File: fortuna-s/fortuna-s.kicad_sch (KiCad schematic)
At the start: 44 parts, among them J1 Ext Pinout, J2 Conn_01x21, J3 Conn_01x21, J6 Power (to panel), U1 74HTC138, U2 74HTC175

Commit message: .
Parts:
- removed C1, C2, C? (x4): 10uF, symbol Device:C
- removed J1: Ext Pinout, symbol Connector_Generic:Conn_02x13_Counter_Clockwise
- removed J2, J3: Conn_01x21, symbol Connector_Generic:Conn_01x21
- removed J?: FTDI cable, symbol Connector_Generic:Conn_01x06
- removed R? (x4): 10K, symbol Device:R_US
- removed R?: 3k3, symbol Device:R_US
- removed U1: 74HTC138, symbol 74xx:74LS138
- removed U2: 74HTC175, symbol 74xx:74LS175
- removed U? (x4): 74LS32, symbol 74xx:74LS32
- removed U?: 28C256, symbol Memory_EEPROM:28C256
- removed U?: AS6C4008-55PCN, Package_DIP:DIP-32_W15.24mm, symbol Memory_RAM:AS6C4008-55PCN
- removed U?: MC68B50, Package_DIP:DIP-40_W15.24mm, symbol Interface_UART:MC68B50
- removed U? (x2): 74HCT04, symbol 74xx:74HCT04
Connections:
- net VCC: no longer P?.A4 (VBUS), P?.A9 (VBUS), P?.B4 (VBUS), P?.B9 (VBUS), SW?.1
- net CLK_UART renamed CLK_EXT
- new net 5V_FTDI: P?.A4 (VBUS), P?.A9 (VBUS), P?.B4 (VBUS), P?.B9 (VBUS), SW?.1
- no-connect marks 18 -> 7
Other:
- added sheet Memory (memory.kicad_sch)
- added sheet Peripheral (peripheral.kicad_sch)
- note removed: "0x80 - Write serial 0x81 - Read serial"
- note removed: "BANKSWITCHING"
- note removed: "DEBUGGER"
- note removed: "EXTERNAL I/O"
- note removed: "I/O MULTIPLEXER"
- note removed: "IO address: write to 0x0"
- note removed: "MEMORY"
- note removed: "Occupies 0x80 to 0xBF in memory map."
- note removed: "The computer can be powered by the FTDI cable, but current can't exceed 350 mA."
- note removed: "UART"
- note removed: "UART communcates at 115000 baud."
- moved on the sheet: C?, D?, J6, JP1, JP?, P?, R?, SW?, U?, X?

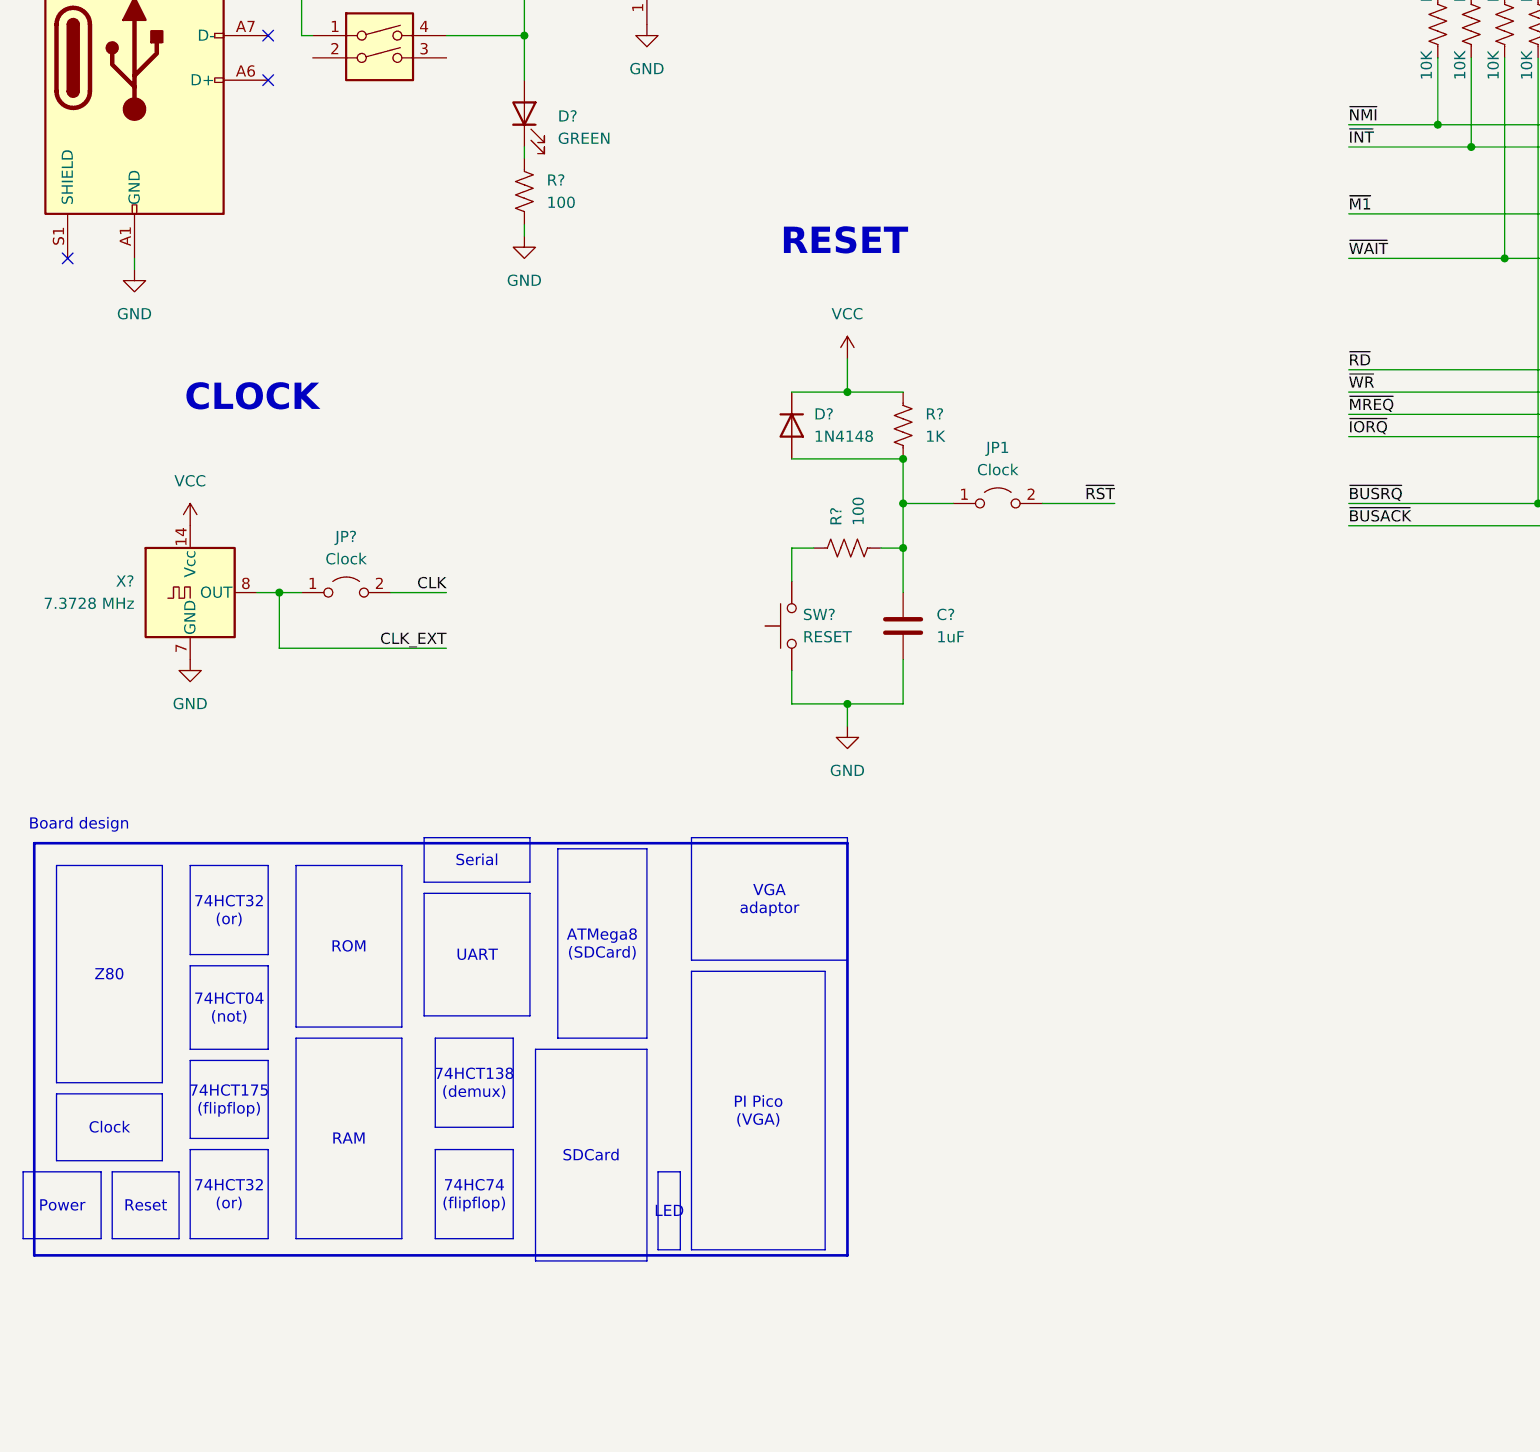
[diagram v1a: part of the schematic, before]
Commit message: .
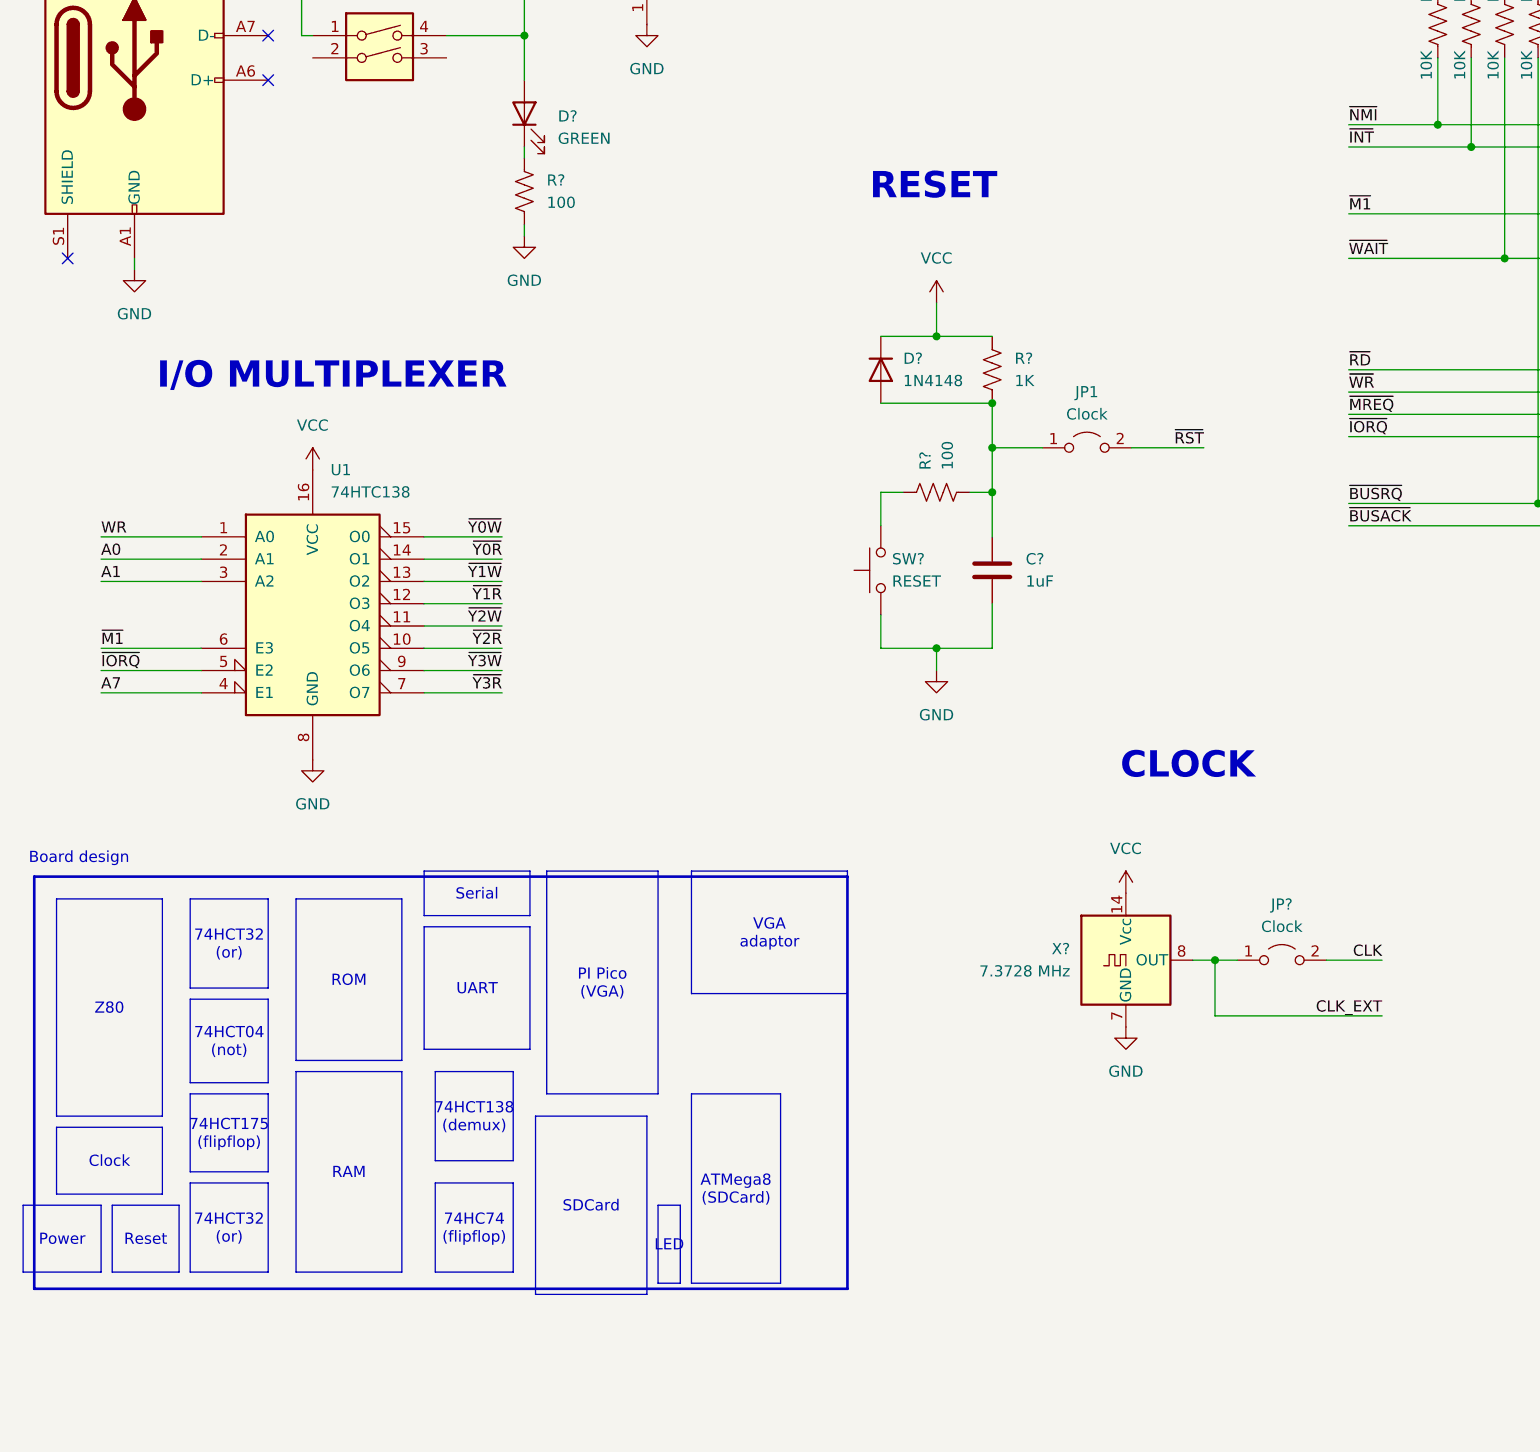
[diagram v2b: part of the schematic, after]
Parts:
- added U1: 74HTC138, symbol 74xx:74LS138
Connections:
- net GND: now also U1.8 (GND)
- net VCC: now also U1.16 (VCC)
- net ~{IORQ}: now also U1.5 (E2)
- net ~{M1}: now also U1.6 (E3)
- new net A0: U1.2 (A1)
- new net A1: U1.3 (A2)
- new net A7: U1.4 (E1)
- new net WR: U1.1 (A0)
- new net ~{Y0R}: U1.14 (O1)
- new net ~{Y0W}: U1.15 (O0)
- new net ~{Y1R}: U1.12 (O3)
- new net ~{Y1W}: U1.13 (O2)
- new net ~{Y2R}: U1.10 (O5)
- new net ~{Y2W}: U1.11 (O4)
- new net ~{Y3R}: U1.7 (O7)
- new net ~{Y3W}: U1.9 (O6)
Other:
- note added: "I/O MULTIPLEXER"
- moved on the sheet: C?, D?, JP1, JP?, R?, SW?, X?

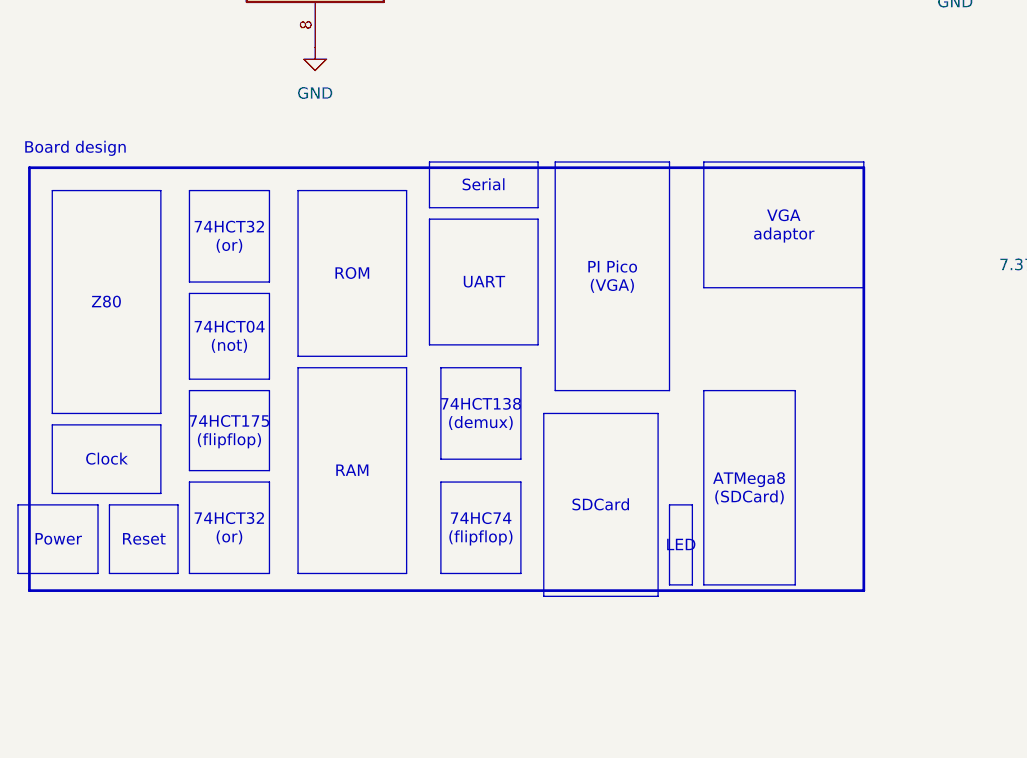
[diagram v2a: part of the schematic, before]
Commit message: .
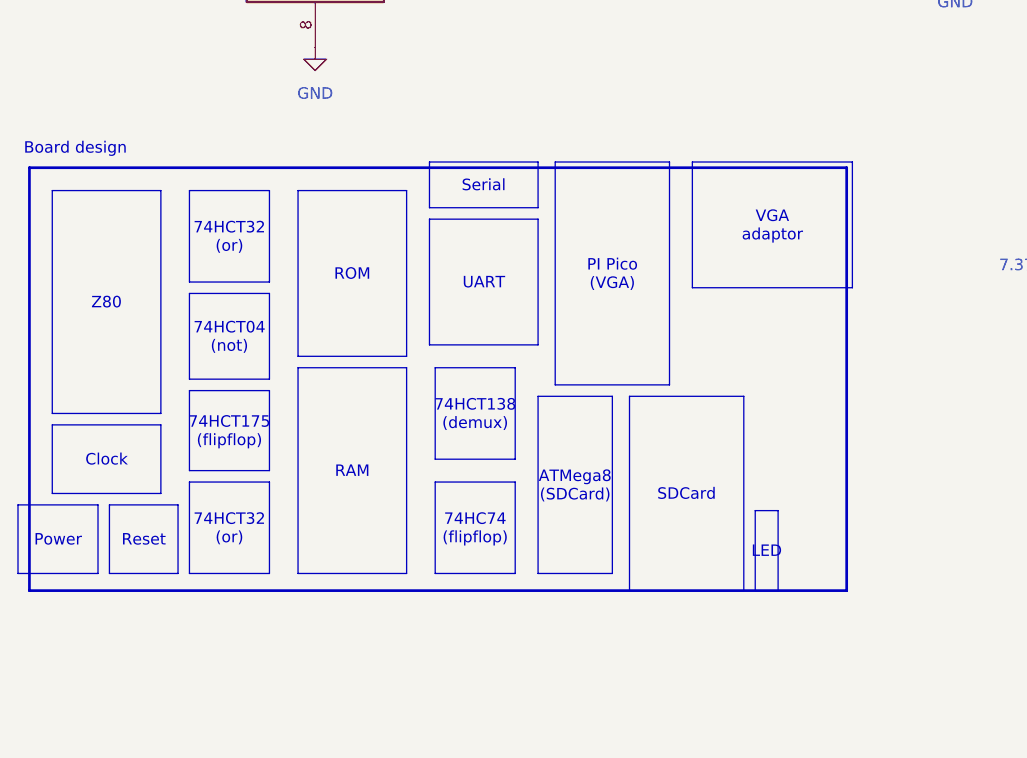
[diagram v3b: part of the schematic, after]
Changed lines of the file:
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@@
     (stroke (width 0) (type default))
   )
-  (rectangle (start 25.4 146.685) (end 118.11 193.675)
+  (rectangle (start 25.4 146.685) (end 116.205 193.675)
     (stroke (width 0.3) (type default))
     (fill (type none))
@@
   )
   (text_box "ATMega8\n(SDCard)"
-    (at 100.33 171.45 0) (size 10.16 21.59)
+    (at 81.915 172.085 0) (size 8.255 19.685)
     (stroke (width 0) (type default))
     (fill (type none))
@@
   )
   (text_box "SDCard"
-    (at 82.55 173.99 0) (size 12.7 20.32)
+    (at 92.075 172.085 0) (size 12.7 21.59)
     (stroke (width 0) (type default))
     (fill (type none))
@@
   )
   (text_box "74HCT138\n(demux)"
-    (at 71.12 168.91 0) (size 8.89 10.16)
+    (at 70.485 168.91 0) (size 8.89 10.16)
     (stroke (width 0) (type default))
     (fill (type none))
@@
   )
   (text_box "VGA\nadaptor"
-    (at 100.33 146.05 0) (size 17.78 13.97)
+    (at 99.06 146.05 0) (size 17.78 13.97)
     (stroke (width 0) (type default))
     (fill (type none))
@@
   )
   (text_box "LED"
-    (at 96.52 184.15 0) (size 2.54 8.89)
+    (at 106.045 184.785 0) (size 2.54 8.89)
     (stroke (width 0) (type default))
     (fill (type none))
@@
   )
   (text_box "PI Pico\n(VGA)"
-    (at 83.82 146.05 0) (size 12.7 25.4)
+    (at 83.82 146.05 0) (size 12.7 24.765)
     (stroke (width 0) (type default))
     (fill (type none))
@@
   )
   (text_box "74HC74\n(flipflop)"
-    (at 71.12 181.61 0) (size 8.89 10.16)
+    (at 70.485 181.61 0) (size 8.89 10.16)
     (stroke (width 0) (type default))
     (fill (type none))
